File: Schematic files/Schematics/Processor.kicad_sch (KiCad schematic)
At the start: 17 parts, among them J6 UV LED Socket, SW1 SW_SPDT, U2 STM32F103C8Tx, Y1 16MHz

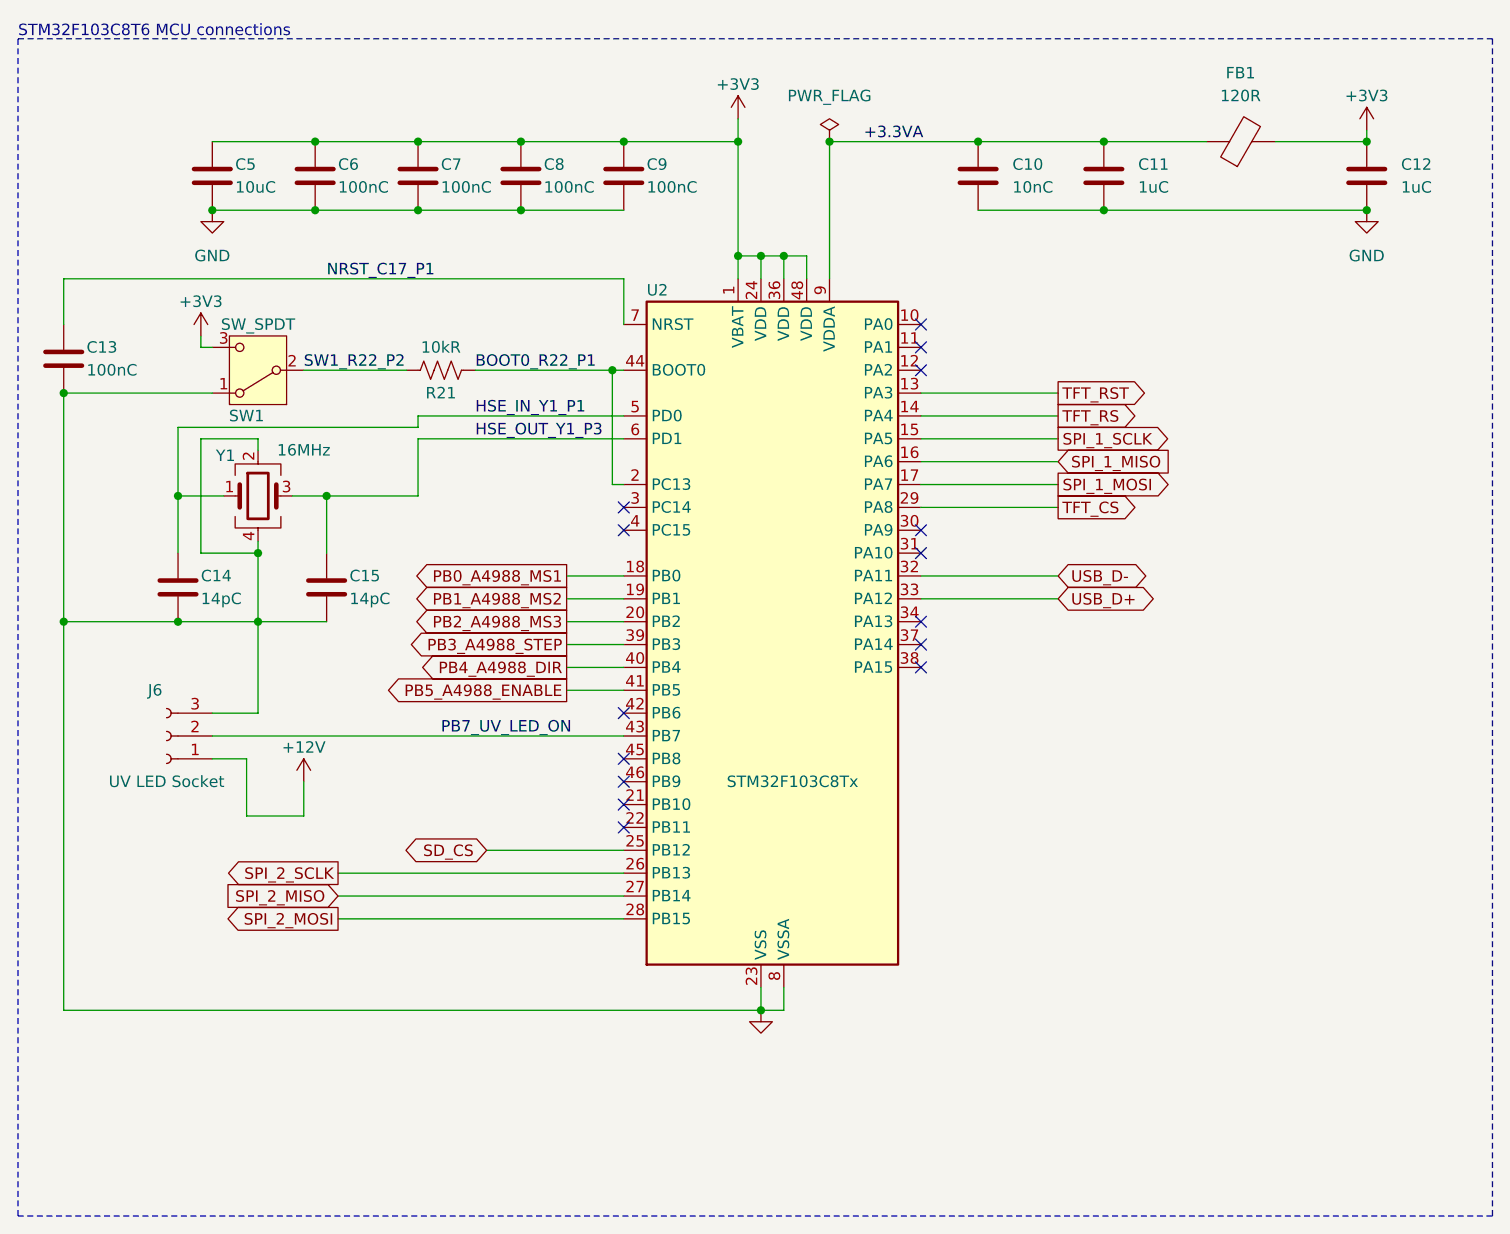
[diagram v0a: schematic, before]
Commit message: pcb
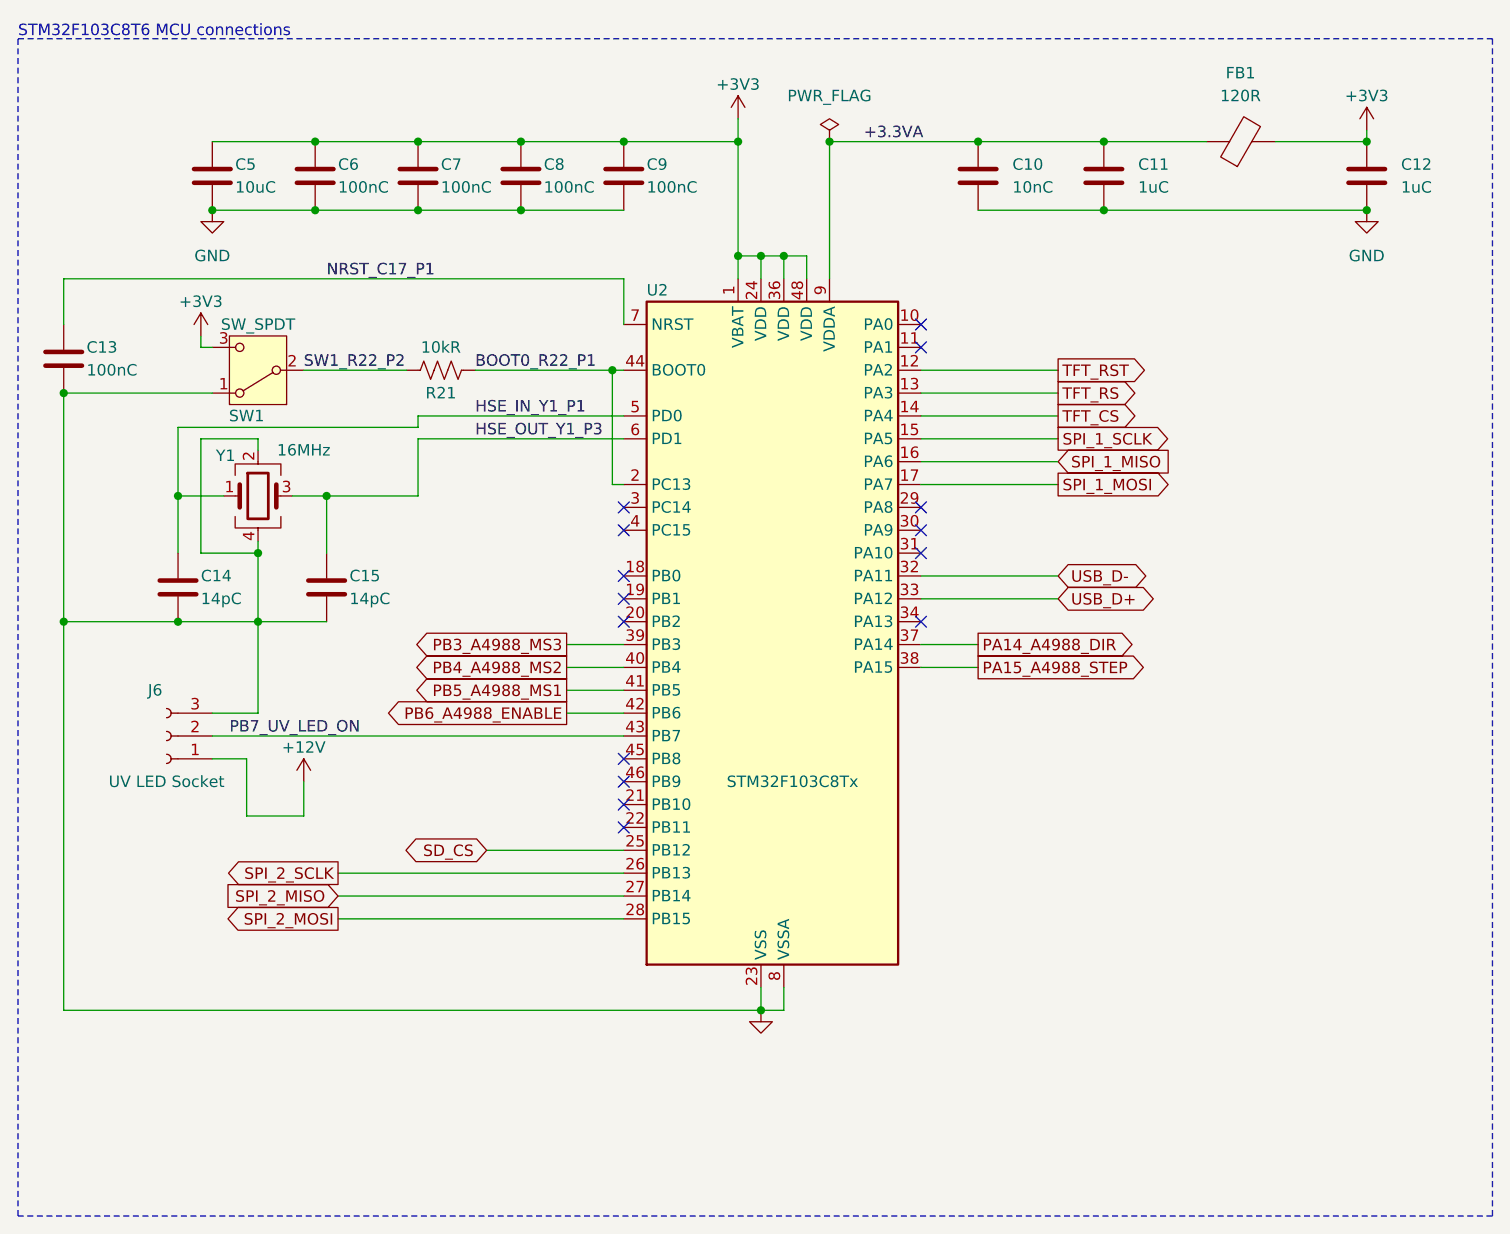
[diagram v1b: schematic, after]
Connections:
- net TFT_CS: now also U2.14 (PA4); no longer U2.29 (PA8)
- net TFT_RS: now also U2.13 (PA3); no longer U2.14 (PA4)
- net TFT_RST: now also U2.12 (PA2); no longer U2.13 (PA3)
- net PA14_A4988_DIR: now reaches U2.37 (PA14)
- net PA15_A4988_STEP: now reaches U2.38 (PA15)
- net PB6_A4988_ENABLE: now reaches U2.42 (PB6)
- net PB0_A4988_MS1: no longer names the net of U2.18 (PB0)
- net PB1_A4988_MS2: no longer names the net of U2.19 (PB1)
- net PB2_A4988_MS3: no longer names the net of U2.20 (PB2)
- net PB3_A4988_STEP renamed PB3_A4988_MS3
- net PB4_A4988_DIR renamed PB4_A4988_MS2
- net PB5_A4988_ENABLE renamed PB5_A4988_MS1
